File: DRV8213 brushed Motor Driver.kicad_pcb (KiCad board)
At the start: 4 copper layers, 15 x 15 mm, 26 parts, among them J1 Keystone 6102, J10 Precidip 852-10-004-20-001101, J11 Precidip 852-10-004-20-001101, J2 Keystone 6102, J3 Keystone 6100, J4 Keystone 6100, J5 Keystone 6102, J6 Keystone 6102, J7 Keystone 6100, J8 Keystone 6100, J9 JST PH 2mm horizontal, U1 DRV8213RTER, U2 LP2981-3.3

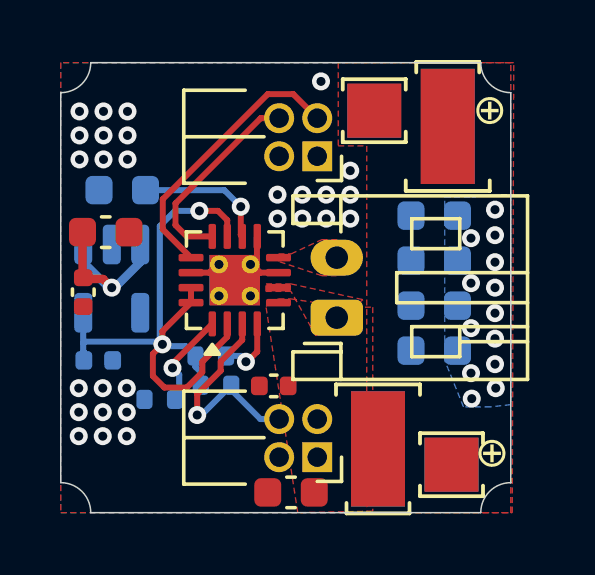
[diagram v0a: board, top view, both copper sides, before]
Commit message: Fixed connector alignment
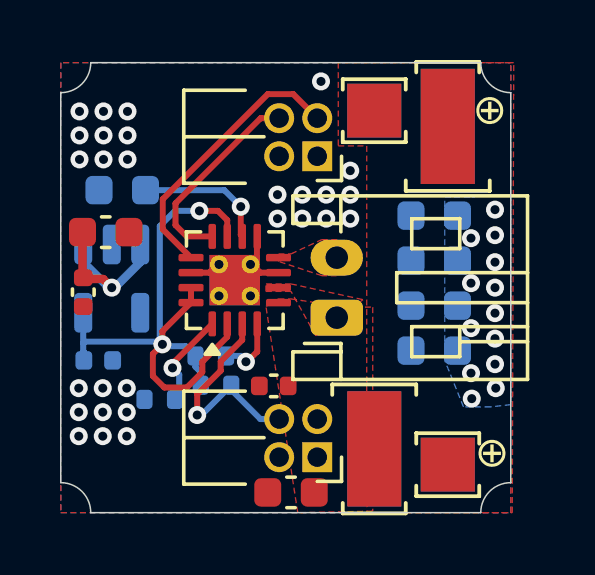
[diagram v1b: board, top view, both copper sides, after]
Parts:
- moved J1 0.12 mm to (174.2, 107.1)
- moved J3 0.12 mm to (176.7, 107.6)
- moved J5 0.12 mm to (174.2, 107.1)
- moved J7 0.12 mm to (176.7, 107.6)
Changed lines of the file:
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@@
 	(footprint "custom_Connector:Keystone_6100"
 		(layer "F.Cu")
-		(at 176.825 107.6)
+		(at 176.7 107.6)
 		(property "Reference" "J3"
 			(at 0.3 -2.55 0)
@@
 	(footprint "custom_Connector:Keystone_6102"
 		(layer "F.Cu")
-		(at 174.375 107.075)
+		(at 174.25 107.075)
 		(property "Reference" "J1"
 			(at 1.9 -0.2 90)
@@
 	(footprint "custom_Connector:Keystone_6102"
 		(layer "B.Cu")
-		(at 174.375 107.075 180)
+		(at 174.25 107.075 180)
 		(property "Reference" "J5"
 			(at 1.9 0.2 90)
@@
 	(footprint "custom_Connector:Keystone_6100"
 		(layer "B.Cu")
-		(at 176.825 107.6 180)
+		(at 176.7 107.6 180)
 		(property "Reference" "J7"
 			(at 0.3 2.55 0)
